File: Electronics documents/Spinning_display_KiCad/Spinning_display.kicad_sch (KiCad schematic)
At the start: 52 parts

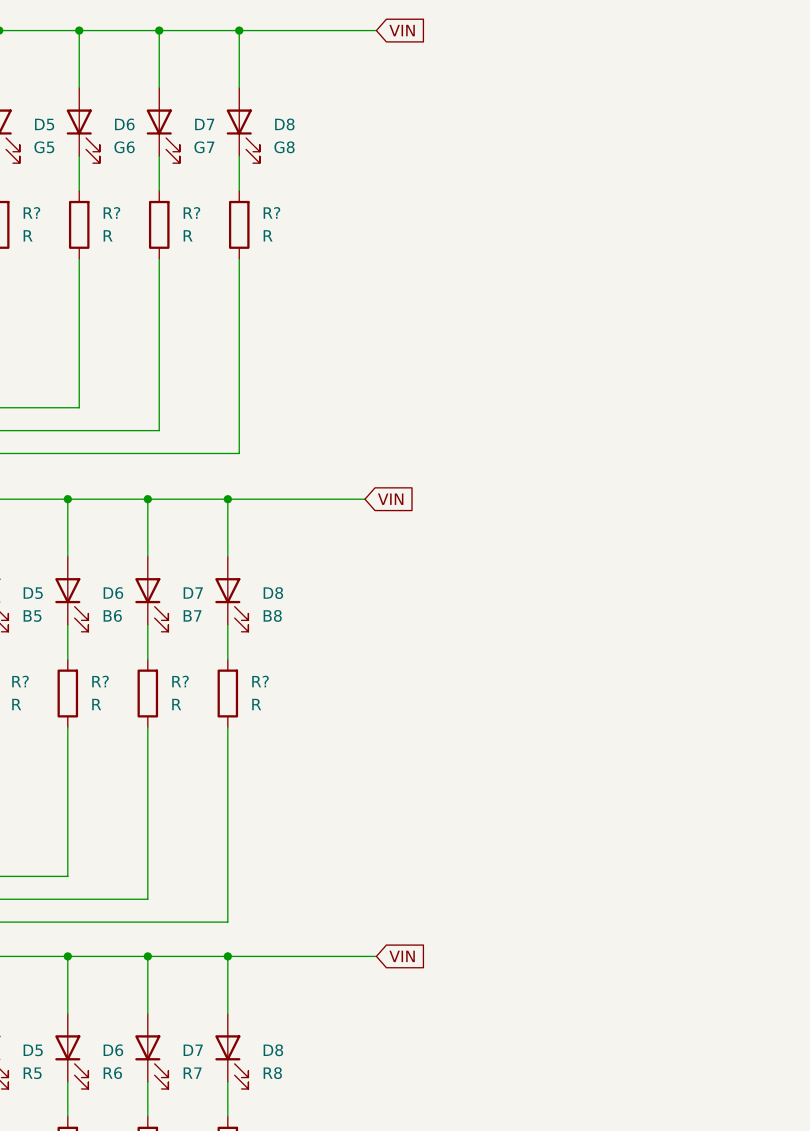
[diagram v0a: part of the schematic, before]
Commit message: Schematics update (common catode instead of anode)
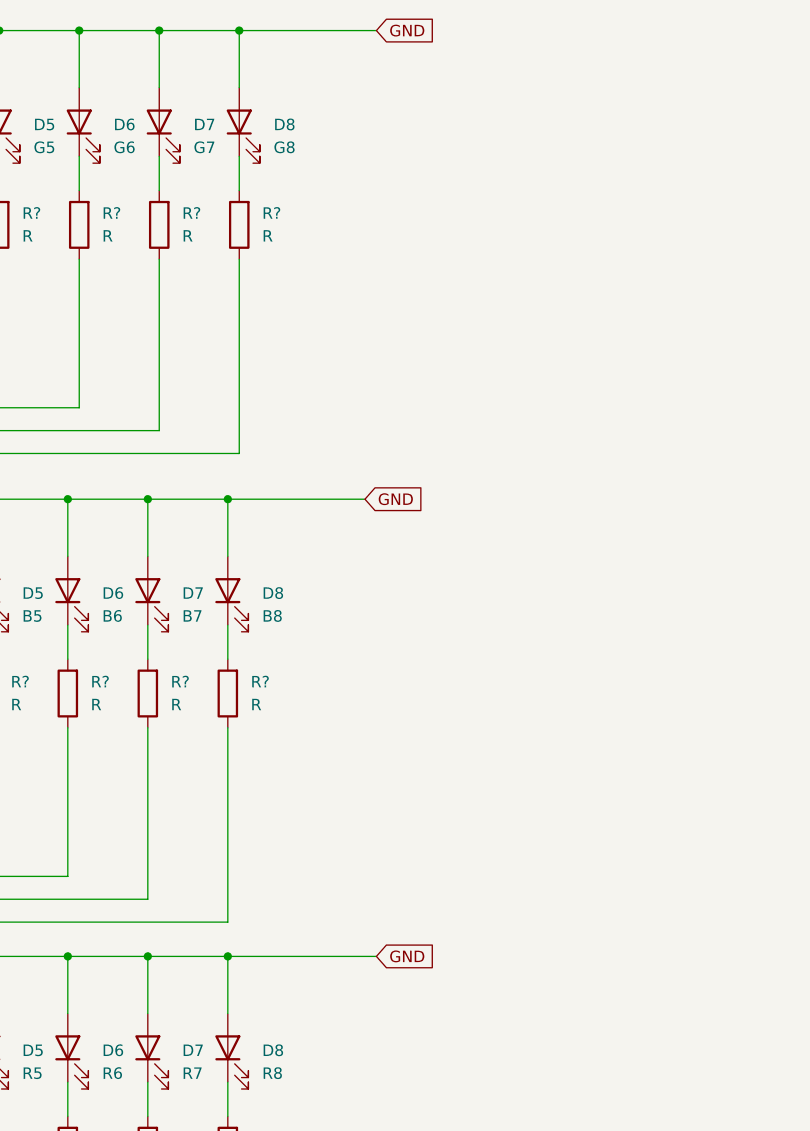
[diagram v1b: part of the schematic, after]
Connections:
- net VIN is gone; now on net GND: D1.2 (A), D1.2 (A), D1.2 (A), D2.2 (A), D2.2 (A), D2.2 (A), D3.2 (A), D3.2 (A), D3.2 (A), D4.2 (A), D4.2 (A), D4.2 (A), D5.2 (A), D5.2 (A), D5.2 (A), D6.2 (A), D6.2 (A), D6.2 (A), D7.2 (A), D7.2 (A), D7.2 (A), D8.2 (A), D8.2 (A), D8.2 (A)
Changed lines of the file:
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@@
     )
   )
-  (global_label "VIN" (shape input) (at 144.78 26.67 0) (fields_autoplaced)
+  (global_label "GND" (shape input) (at 144.78 26.67 0) (fields_autoplaced)
     (effects (font (size 1.27 1.27)) (justify left))
-    (property "Intersheet References" "${INTERSHEET_REFS}" (id 0) (at 150.2169 26.5906 0)
+    (property "Intersheet References" "${INTERSHEET_REFS}" (id 0) (at 151.0636 26.5906 0)
       (effects (font (size 1.27 1.27)) (justify left) hide)
     )
@@
     )
   )
-  (global_label "VIN" (shape input) (at 144.78 129.54 0) (fields_autoplaced)
+  (global_label "GND" (shape input) (at 144.78 129.54 0) (fields_autoplaced)
     (effects (font (size 1.27 1.27)) (justify left))
-    (property "Intersheet References" "${INTERSHEET_REFS}" (id 0) (at 150.2169 129.4606 0)
+    (property "Intersheet References" "${INTERSHEET_REFS}" (id 0) (at 151.0636 129.4606 0)
       (effects (font (size 1.27 1.27)) (justify left) hide)
     )
@@
     )
   )
-  (global_label "VIN" (shape input) (at 143.51 78.74 0) (fields_autoplaced)
+  (global_label "GND" (shape input) (at 143.51 78.74 0) (fields_autoplaced)
     (effects (font (size 1.27 1.27)) (justify left))
-    (property "Intersheet References" "${INTERSHEET_REFS}" (id 0) (at 148.9469 78.6606 0)
+    (property "Intersheet References" "${INTERSHEET_REFS}" (id 0) (at 149.7936 78.6606 0)
       (effects (font (size 1.27 1.27)) (justify left) hide)
     )

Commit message: COMMON ANODE i was mistaken
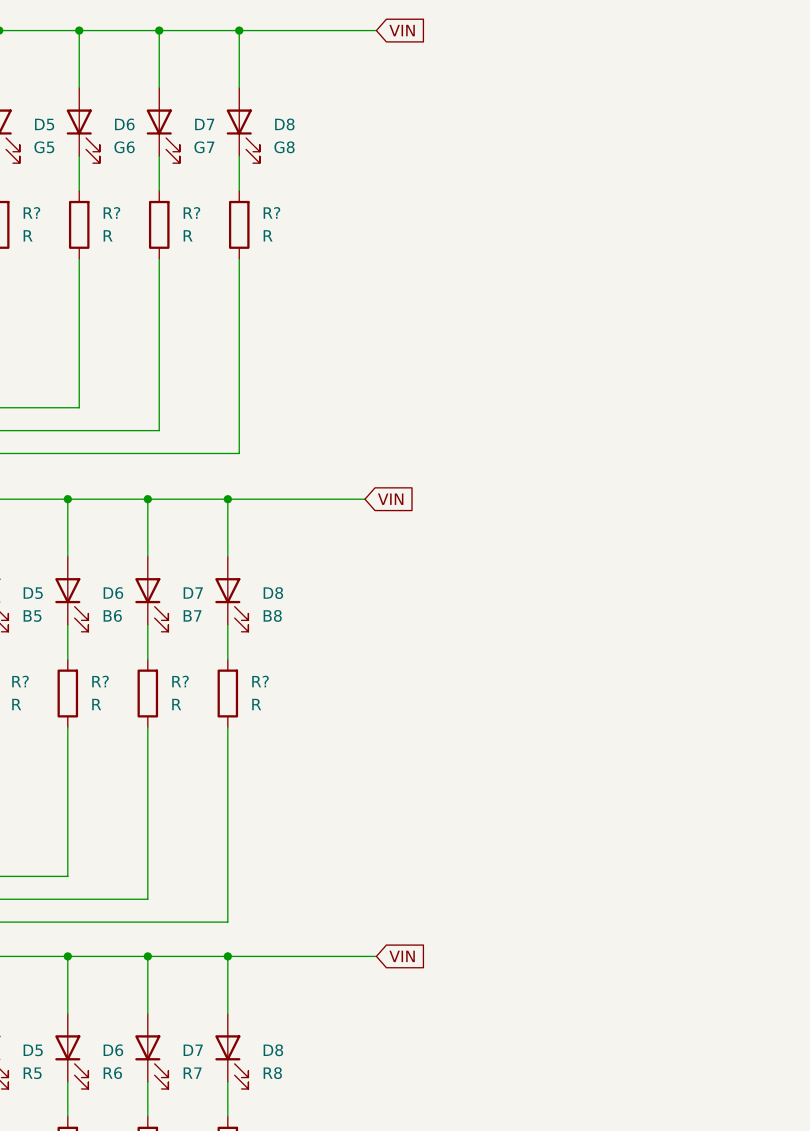
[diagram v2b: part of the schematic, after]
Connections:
- net GND: no longer D1.2 (A), D1.2 (A), D1.2 (A), D2.2 (A), D2.2 (A), D2.2 (A), D3.2 (A), D3.2 (A), D3.2 (A), D4.2 (A), D4.2 (A), D4.2 (A), D5.2 (A), D5.2 (A), D5.2 (A), D6.2 (A), D6.2 (A), D6.2 (A), D7.2 (A), D7.2 (A), D7.2 (A), D8.2 (A), D8.2 (A), D8.2 (A)
- new net VIN: D1.2 (A), D1.2 (A), D1.2 (A), D2.2 (A), D2.2 (A), D2.2 (A), D3.2 (A), D3.2 (A), D3.2 (A), D4.2 (A), D4.2 (A), D4.2 (A), D5.2 (A), D5.2 (A), D5.2 (A), D6.2 (A), D6.2 (A), D6.2 (A), D7.2 (A), D7.2 (A), D7.2 (A), D8.2 (A), D8.2 (A), D8.2 (A)
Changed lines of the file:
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@@
     )
   )
-  (global_label "GND" (shape input) (at 144.78 26.67 0) (fields_autoplaced)
+  (global_label "VIN" (shape input) (at 144.78 26.67 0) (fields_autoplaced)
     (effects (font (size 1.27 1.27)) (justify left))
-    (property "Intersheet References" "${INTERSHEET_REFS}" (id 0) (at 151.0636 26.5906 0)
+    (property "Intersheet References" "${INTERSHEET_REFS}" (id 0) (at 150.2169 26.5906 0)
       (effects (font (size 1.27 1.27)) (justify left) hide)
     )
@@
     )
   )
-  (global_label "GND" (shape input) (at 144.78 129.54 0) (fields_autoplaced)
+  (global_label "VIN" (shape input) (at 144.78 129.54 0) (fields_autoplaced)
     (effects (font (size 1.27 1.27)) (justify left))
-    (property "Intersheet References" "${INTERSHEET_REFS}" (id 0) (at 151.0636 129.4606 0)
+    (property "Intersheet References" "${INTERSHEET_REFS}" (id 0) (at 150.2169 129.4606 0)
       (effects (font (size 1.27 1.27)) (justify left) hide)
     )
@@
     )
   )
-  (global_label "GND" (shape input) (at 143.51 78.74 0) (fields_autoplaced)
+  (global_label "VIN" (shape input) (at 143.51 78.74 0) (fields_autoplaced)
     (effects (font (size 1.27 1.27)) (justify left))
-    (property "Intersheet References" "${INTERSHEET_REFS}" (id 0) (at 149.7936 78.6606 0)
+    (property "Intersheet References" "${INTERSHEET_REFS}" (id 0) (at 148.9469 78.6606 0)
       (effects (font (size 1.27 1.27)) (justify left) hide)
     )
